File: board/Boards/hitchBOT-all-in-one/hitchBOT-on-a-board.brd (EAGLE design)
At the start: 100 x 55 mm, 40 parts, among them J1 22-27-2021-02, J2 22-27-2021-02, J3 22-27-2021-02, Q1 SPD30P06PTO252, Q2 SPD30P06PTO252, Q3 SPD30P06PTO252

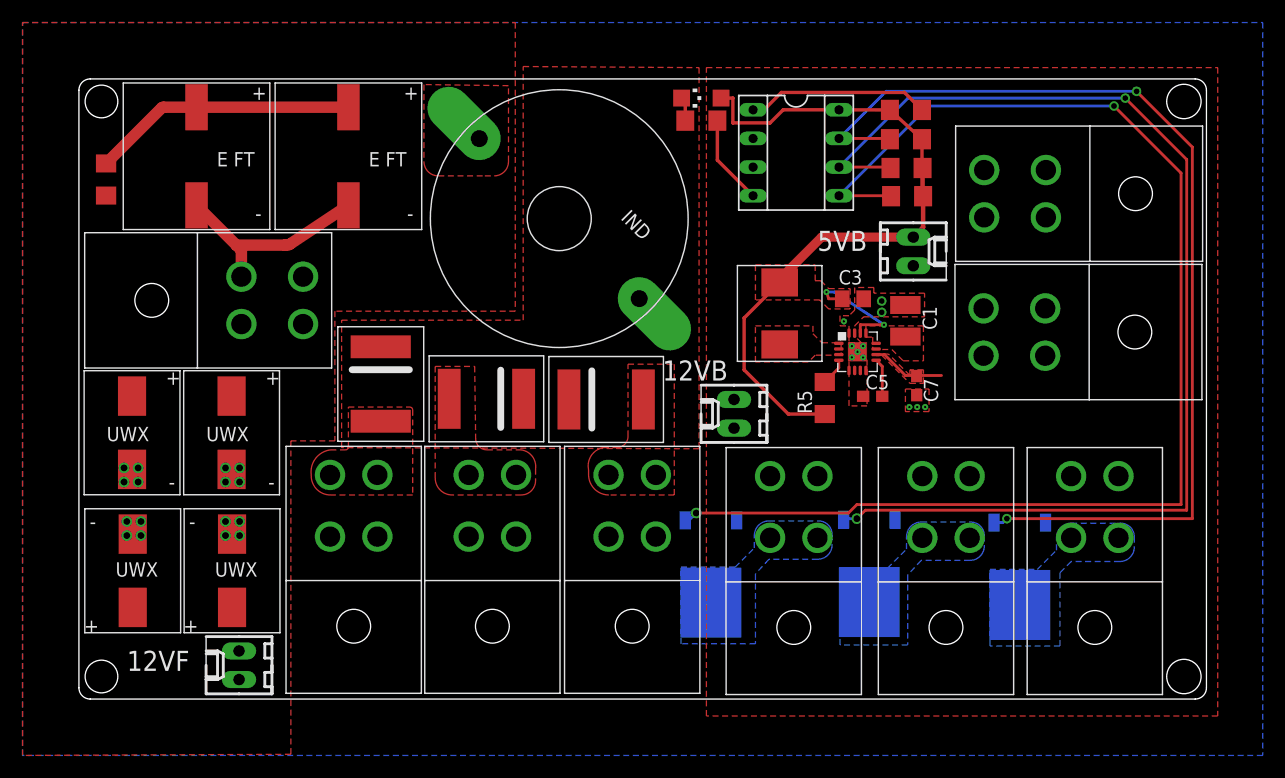
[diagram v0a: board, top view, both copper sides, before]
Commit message: finalized board, what was ordered
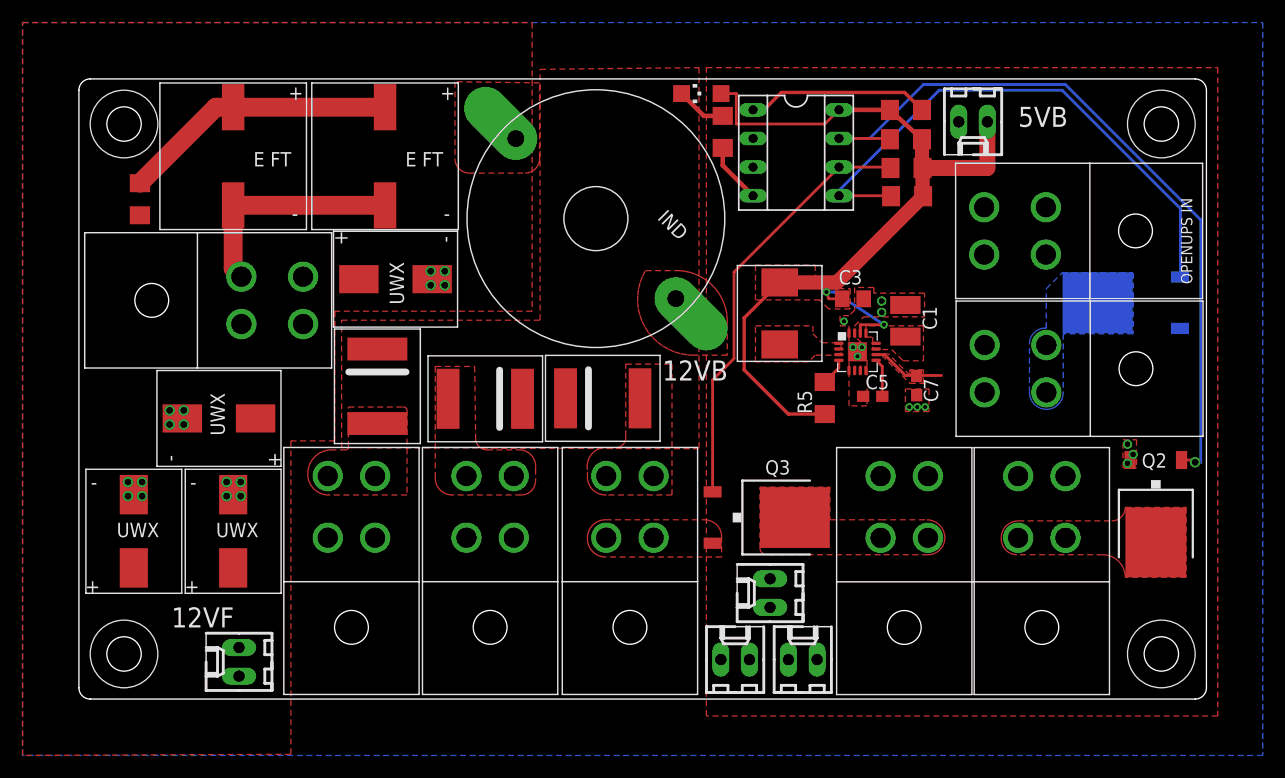
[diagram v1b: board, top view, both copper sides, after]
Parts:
- removed U$16: 2X2-MOLEX, Molex:2X2MOLEX
- added J4, J5: 22-27-2021-02, con-molex:6410-02
- moved Q1 44.0 mm to (92.8, 35.1), turned to 270 degrees
- moved U$13 24.1 mm to (83.7, 29.3), turned to 90 degrees
- moved J3 22.6 mm to (64.2, 3.50), turned to 0 degrees
- moved C13 19.9 mm to (28.1, 37.2), turned to 90 degrees
- moved Q2 13.3 mm to (95.5, 16.4), flipped to the top
- moved J1 12.7 mm to (79.3, 51.2), turned to 180 degrees
- moved Q3 10.4 mm to (61.0, 16.1), flipped to the top, turned to 270 degrees
- moved C11 7.81 mm to (12.4, 24.9), turned to 270 degrees
- moved U$12 4.70 mm to (85.4, 16.4)
- moved U$17 3.70 mm to (73.2, 16.4)
- moved C12 3.50 mm to (13.7, 14.9)
- moved C14 3.50 mm to (4.87, 14.9)
- moved R1 3.47 mm to (5.41, 44.3)
- moved U$11 3.30 mm to (83.7, 41.5)
- moved U$1 3.25 mm to (13.7, 48.1)
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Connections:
- net GND: now also J4.1, J5.1; no longer U$16.GNDL, U$16.GNDR
- net N$8: now also J4.2, J5.2; no longer U$16.POWERL, U$16.POWERR
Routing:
- net N$13: track 114.7 -> 49.5 mm, vias 2 -> 0
- net N$19: track 102.1 -> 38.0 mm, vias 2 -> 0
- net N$11: track 90.3 -> 67.0 mm, vias 2 -> 1
- net N$15: track 72.8 -> 82.7 mm
- net N$20: track 2.33 -> 4.47 mm
- net GND: track 29.3 -> 27.9 mm, vias 27 -> 28
- net N$2: track 23.5 -> 24.5 mm
- added copper zone on layer 1, net N$10
- added copper zone on layer 1, net N$18
- removed copper zone on layer 16, net N$10
- removed copper zone on layer 16, net N$18
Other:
- board text removed: "UNSWITCHED 12V"
